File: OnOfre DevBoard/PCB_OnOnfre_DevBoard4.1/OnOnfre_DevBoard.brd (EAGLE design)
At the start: 44.7 x 44.5 mm, 27 parts, among them J3Y S8050, J7 8p, K1 OMRON-G3MB-202P-SSR2, K2 OMRON-G3MB-202P-SSR2, U2 esp12

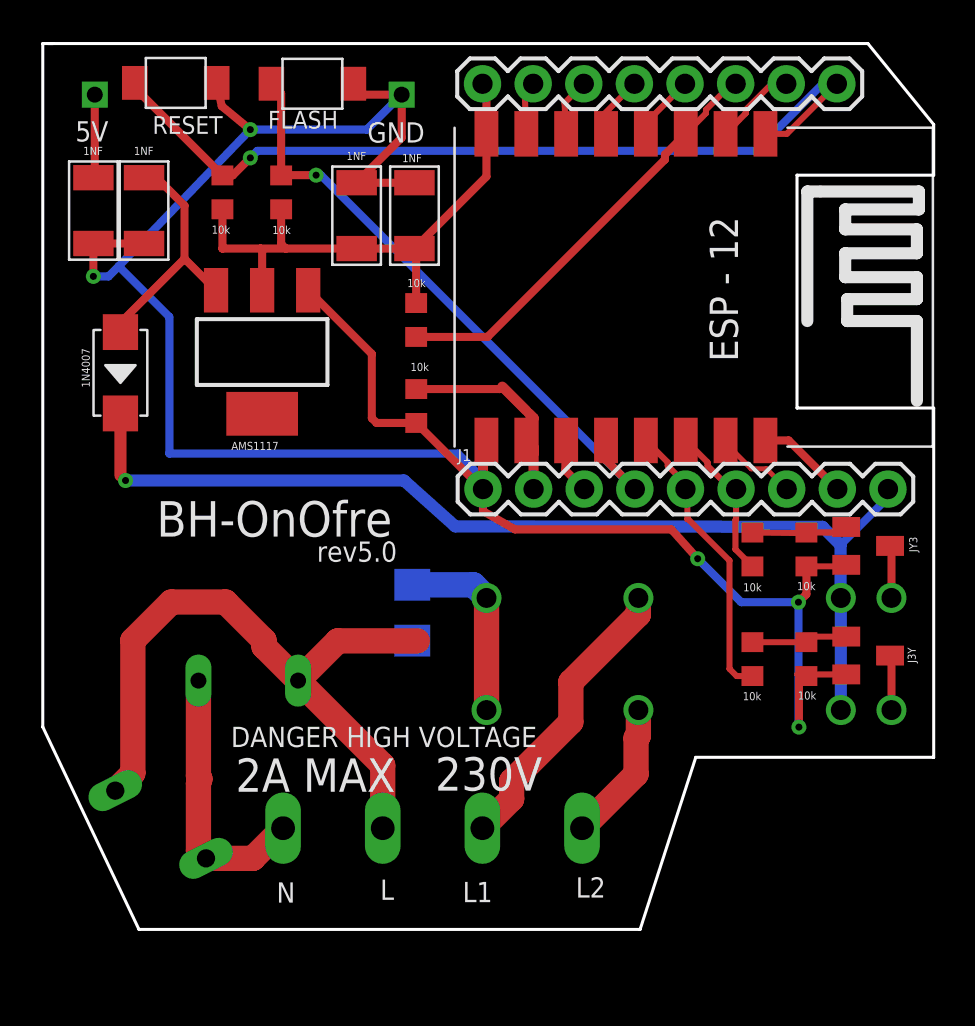
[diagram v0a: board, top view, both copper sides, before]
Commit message: Revert "rev5.0dev"
This reverts commit 2e2358a8c57761c3fa030a0a65c911856fe9a90b.
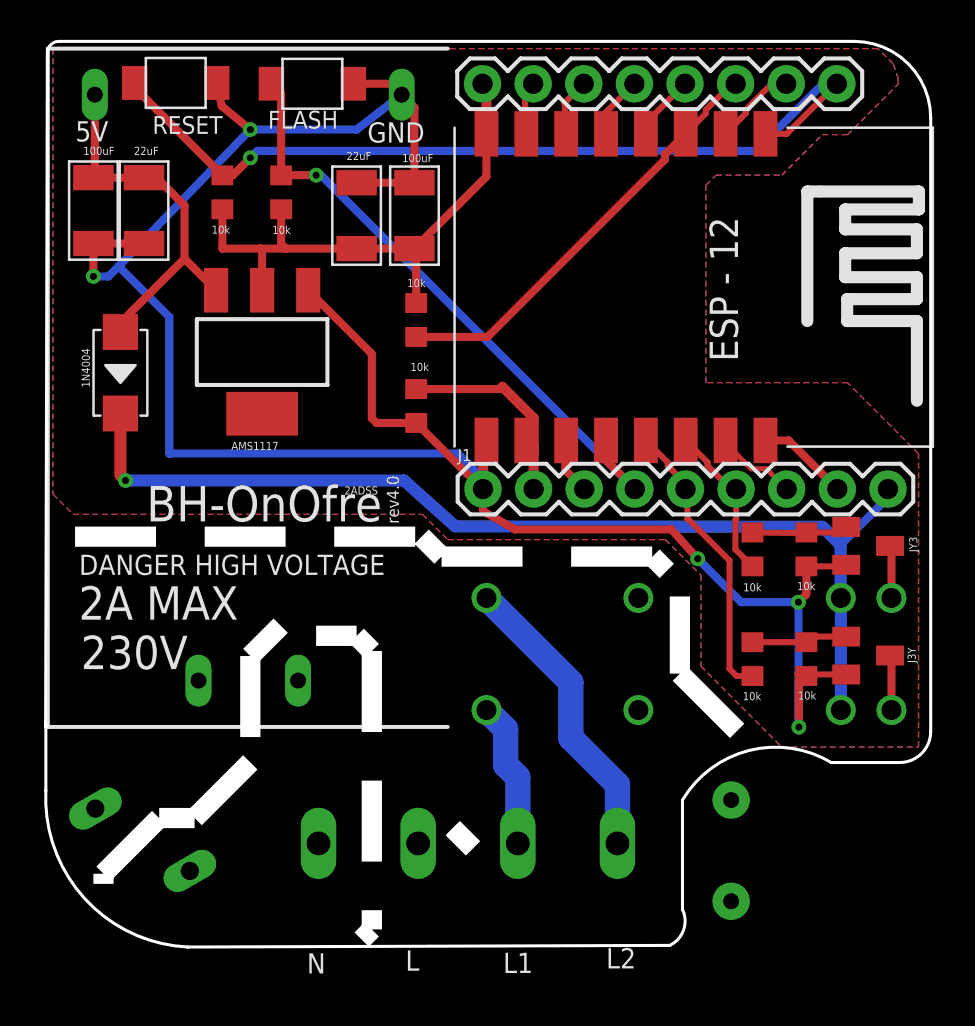
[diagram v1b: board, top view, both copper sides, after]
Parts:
- C1, C2: value 1NF -> 22uF
- C3, C4: value 1NF -> 100uF
- D3: value 1N4007 -> 1N4004
- F1: value 6V/0.75A -> FUSE 2A; device SparkFun-Fuses:1206 -> SparkFun-Fuses:PTH
- R5: value 10D391K 390V -> VARISTORS07K230
- moved F1 20.0 mm to (34.8, 5.73)
- moved X1 1.93 mm to (21.6, 4.83)
- moved R5 1.18 mm to (5.26, 6.28), turned to 330 degrees
- flipped U$2 to the bottom
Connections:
- removed net LIVE: F1.1, R5.1, U$2.P$2, X1.2
- removed net LIVE_FUSED: F1.2, K1.1, K2.1
- removed net LIVE_ONE_OUT: K2.2, X1.3
- removed net LIVE_TWO_OUT: K1.2, X1.4
- removed net N$2: U2.VCC
- removed net NEUTRAL: R5.2, U$2.P$1, X1.1
- new net FASE_IN: R5.1, U$2.P$1, X1.1
- new net NEUTRAL_IN: F1.P$1, R5.2, U$2.P$2, X1.2
- new net NEUTRAL_IN_FUSED: F1.P$2, K1.2, K2.2
- new net NEUTRAL_ONE_OUT: K1.1, X1.3
- new net NEUTRAL_TWO_OUT: K2.1, X1.4
- net 3V3: now also U2.VCC
- net GND: now also U$2.P$3; no longer U$2.P$4
- net VCC: now also U$2.P$4; no longer U$2.P$3
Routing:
- net LIVE: track 34.8 -> 0.00 mm
- net NEUTRAL_TWO_OUT: track 0.00 -> 15.0 mm
- net LIVE_ONE_OUT: track 14.8 -> 0.00 mm
- net NEUTRAL: track 13.6 -> 0.00 mm
- net LIVE_FUSED: track 9.62 -> 0.00 mm
- net NEUTRAL_ONE_OUT: track 0.00 -> 7.34 mm
- net LIVE_TWO_OUT: track 7.10 -> 0.00 mm
- net VCC: track 16.7 -> 19.3 mm
- net 3V3: track 28.4 -> 30.7 mm
- net GND: track 116.7 -> 115.9 mm
- added copper zone on layer 1, net GND
- added copper zone on layer 16, net GND
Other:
- board size 44.7 x 44.5 mm -> 44.4 x 45.4 mm
- board text added: "2ADSS"
- board text added: "HLK-PM01"
- board text added: "rev4.0"
- board text removed: "rev5.0"

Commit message: rev5.0dev
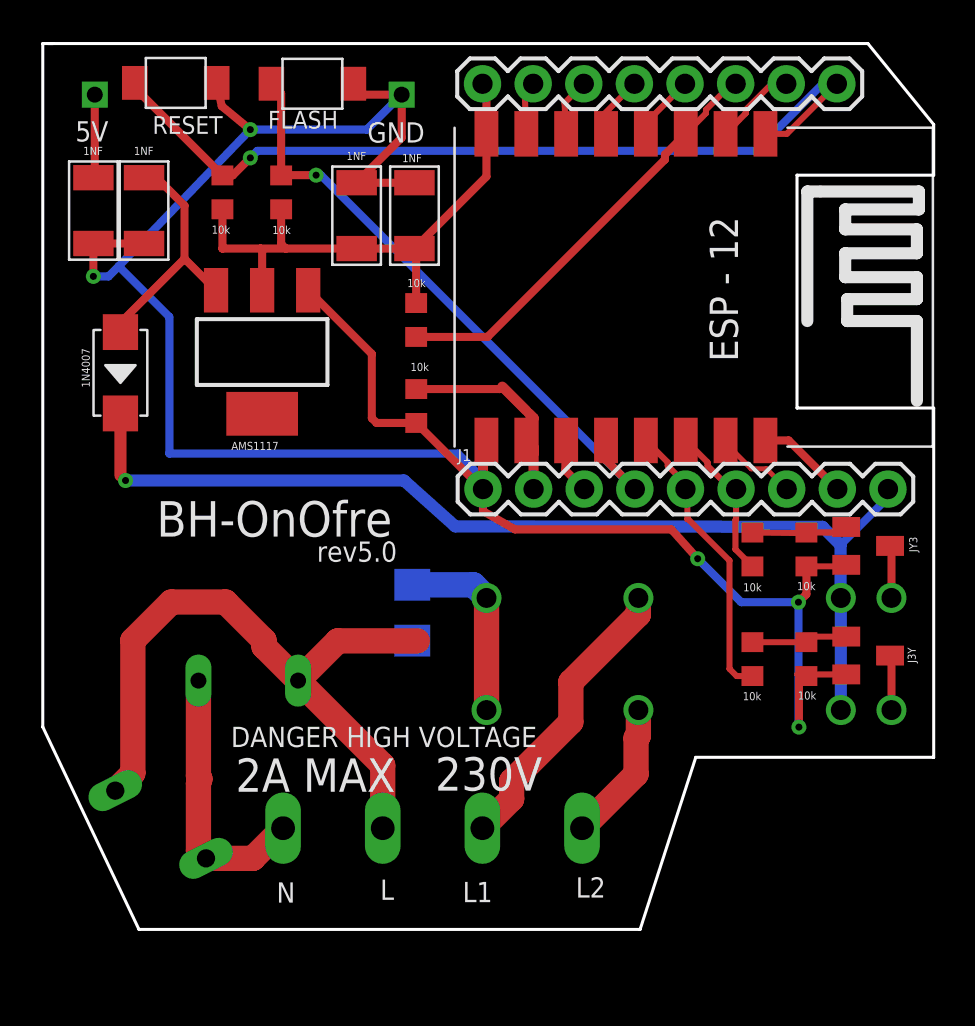
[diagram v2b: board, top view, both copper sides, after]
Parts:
- C1, C2: value 22uF -> 1NF
- C3, C4: value 100uF -> 1NF
- D3: value 1N4004 -> 1N4007
- F1: value FUSE 2A -> 6V/0.75A; device SparkFun-Fuses:PTH -> SparkFun-Fuses:1206
- R5: value VARISTORS07K230 -> 10D391K 390V
- moved F1 20.0 mm to (18.8, 17.7)
- moved X1 1.93 mm to (19.8, 5.59)
- moved R5 1.18 mm to (6.17, 7.04), turned to 153.3 degrees
- flipped U$2 to the top
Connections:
- removed net FASE_IN: R5.1, U$2.P$1, X1.1
- removed net NEUTRAL_IN: F1.P$1, R5.2, U$2.P$2, X1.2
- removed net NEUTRAL_IN_FUSED: F1.P$2, K1.2, K2.2
- removed net NEUTRAL_ONE_OUT: K1.1, X1.3
- removed net NEUTRAL_TWO_OUT: K2.1, X1.4
- new net LIVE: F1.1, R5.1, U$2.P$2, X1.2
- new net LIVE_FUSED: F1.2, K1.1, K2.1
- new net LIVE_ONE_OUT: K2.2, X1.3
- new net LIVE_TWO_OUT: K1.2, X1.4
- new net N$2: U2.VCC
- new net NEUTRAL: R5.2, U$2.P$1, X1.1
- net 3V3: no longer U2.VCC
- net GND: now also U$2.P$4; no longer U$2.P$3
- net VCC: now also U$2.P$3; no longer U$2.P$4
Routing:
- net LIVE: track 0.00 -> 34.8 mm
- net NEUTRAL_TWO_OUT: track 15.0 -> 0.00 mm
- net LIVE_ONE_OUT: track 0.00 -> 14.8 mm
- net NEUTRAL: track 0.00 -> 13.6 mm
- net LIVE_FUSED: track 0.00 -> 9.62 mm
- net NEUTRAL_ONE_OUT: track 7.34 -> 0.00 mm
- net LIVE_TWO_OUT: track 0.00 -> 7.10 mm
- net VCC: track 19.3 -> 16.7 mm
- net 3V3: track 30.7 -> 28.4 mm
- net GND: track 115.9 -> 116.7 mm
- removed copper zone on layer 1, net GND
- removed copper zone on layer 16, net GND
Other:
- board size 44.4 x 45.4 mm -> 44.7 x 44.5 mm
- board text added: "rev5.0"
- board text removed: "2ADSS"
- board text removed: "HLK-PM01"
- board text removed: "rev4.0"
